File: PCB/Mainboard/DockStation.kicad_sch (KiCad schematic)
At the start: 99 parts, among them J13 Docking Station, Q24 MUN2114, Q25 BH, Q32 8B, Q33 BH, Q34 BH, U1 EA, U2 7W32, U20 7W14, U26 7W126, U3 HSDL-1000 X03, U57 SN74LVT125, U64 74LV126, U71 SN74LV32

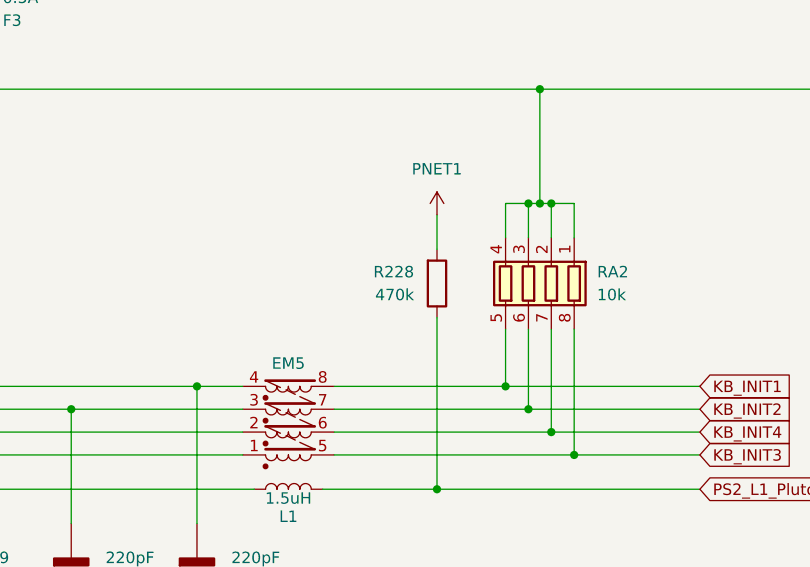
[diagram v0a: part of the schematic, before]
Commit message: Add files via upload
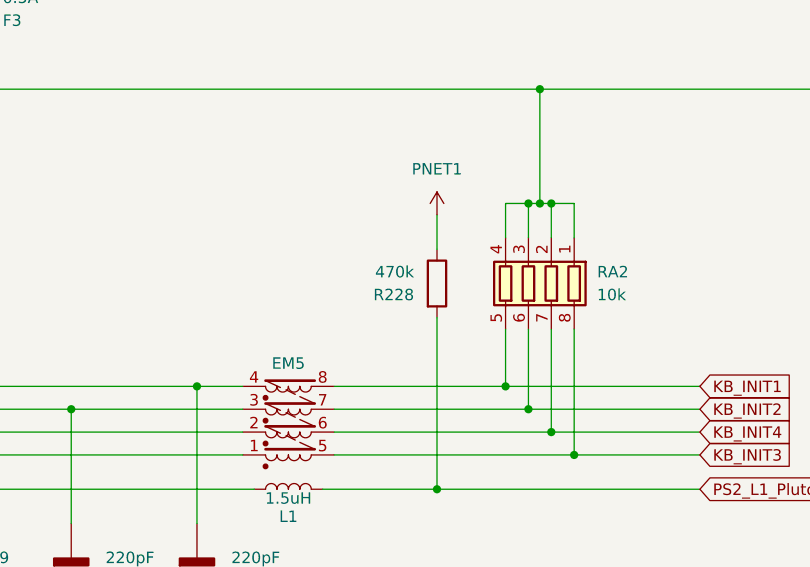
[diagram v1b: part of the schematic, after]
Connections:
- net PNET1: now also R228.1; no longer R228.2
- net PS2_L1_Pluto: now also R228.2; no longer R228.1
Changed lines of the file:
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@@
 		(lib_id "Device:R")
 		(at 281.94 135.89 0)
-		(mirror x)
 		(unit 1)
 		(exclude_from_sim no)
@@
 		(dnp no)
 		(property "Reference" "R228"
-			(at 279.4 134.6199 0)
+			(at 279.4 137.1601 0)
 			(effects
 				(font
@@
 		)
 		(property "Value" "470k"
-			(at 279.4 137.1599 0)
+			(at 279.4 134.6201 0)
 			(effects
 				(font

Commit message: Add files via upload
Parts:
- D52, D53, D54, D56, D57: footprint Package_TO_SOT_SMD:SOT-323_SC-70 -> Package_TO_SOT_SMD:SOT-416
- Q25, Q33, Q34: footprint (none) -> Package_TO_SOT_SMD:SOT-89-3
- Q32: footprint (none) -> Package_TO_SOT_SMD:SOT-416
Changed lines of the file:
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@@
 			)
 		)
-		(property "Footprint" "Package_TO_SOT_SMD:SOT-323_SC-70"
+		(property "Footprint" "Package_TO_SOT_SMD:SOT-416"
 			(at 525.145 520.065 0)
 			(effects
@@
 			)
 		)
-		(property "Footprint" ""
+		(property "Footprint" "Package_TO_SOT_SMD:SOT-89-3"
 			(at 452.12 59.69 0)
 			(effects
@@
 			)
 		)
-		(property "Footprint" "Package_TO_SOT_SMD:SOT-323_SC-70"
+		(property "Footprint" "Package_TO_SOT_SMD:SOT-416"
 			(at 596.265 484.505 0)
 			(effects
@@
 			)
 		)
-		(property "Footprint" ""
+		(property "Footprint" "Package_TO_SOT_SMD:SOT-416"
 			(at 421.64 257.81 0)
 			(effects
@@
 			)
 		)
-		(property "Footprint" "Package_TO_SOT_SMD:SOT-323_SC-70"
+		(property "Footprint" "Package_TO_SOT_SMD:SOT-416"
 			(at 551.815 484.505 0)
 			(effects
@@
 			)
 		)
-		(property "Footprint" ""
+		(property "Footprint" "Package_TO_SOT_SMD:SOT-89-3"
 			(at 228.6 81.28 0)
 			(effects
@@
 			)
 		)
-		(property "Footprint" ""
+		(property "Footprint" "Package_TO_SOT_SMD:SOT-89-3"
 			(at 363.22 251.46 0)
 			(effects
@@
 			)
 		)
-		(property "Footprint" "Package_TO_SOT_SMD:SOT-323_SC-70"
+		(property "Footprint" "Package_TO_SOT_SMD:SOT-416"
 			(at 504.825 484.505 0)
 			(effects
@@
 			)
 		)
-		(property "Footprint" "Package_TO_SOT_SMD:SOT-323_SC-70"
+		(property "Footprint" "Package_TO_SOT_SMD:SOT-416"
 			(at 572.135 520.065 0)
 			(effects
